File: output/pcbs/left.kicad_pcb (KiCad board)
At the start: 2 copper layers, 147 x 117.2 mm, 85 parts

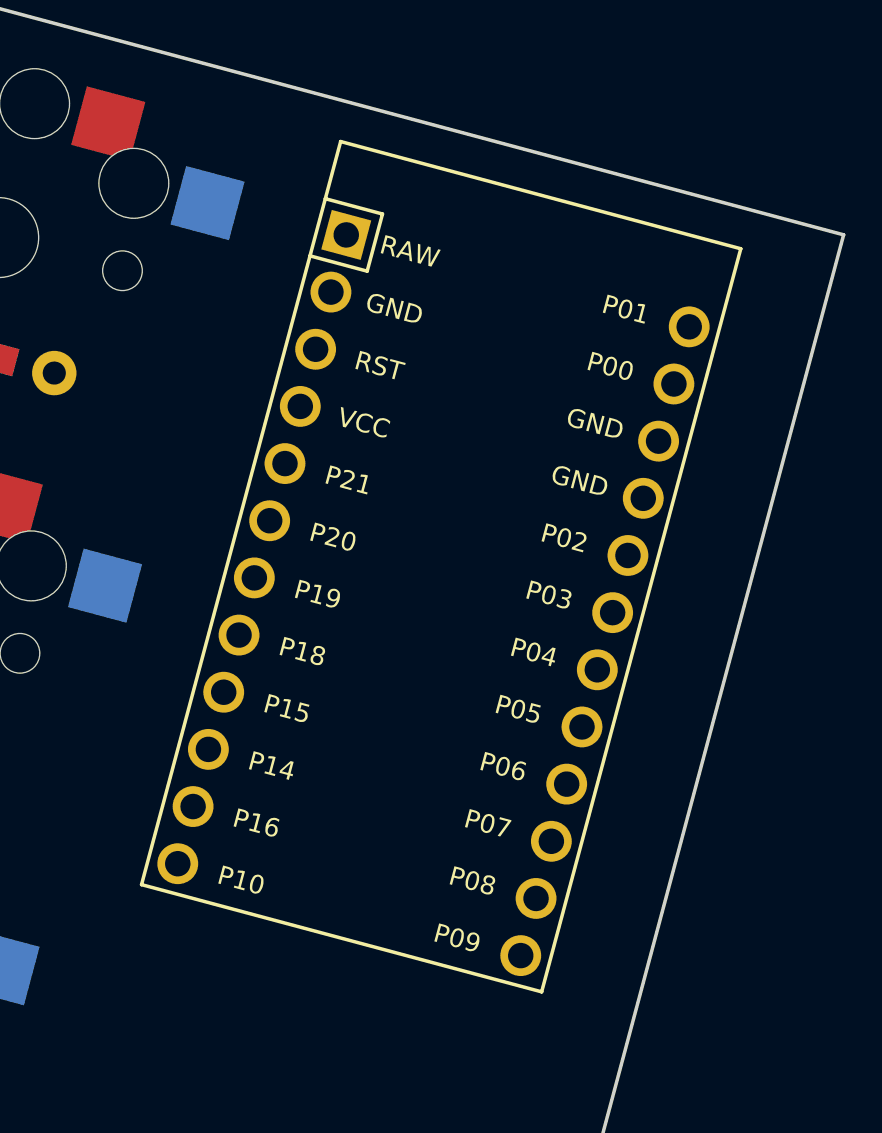
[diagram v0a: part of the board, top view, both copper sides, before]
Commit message: add nrf footprint
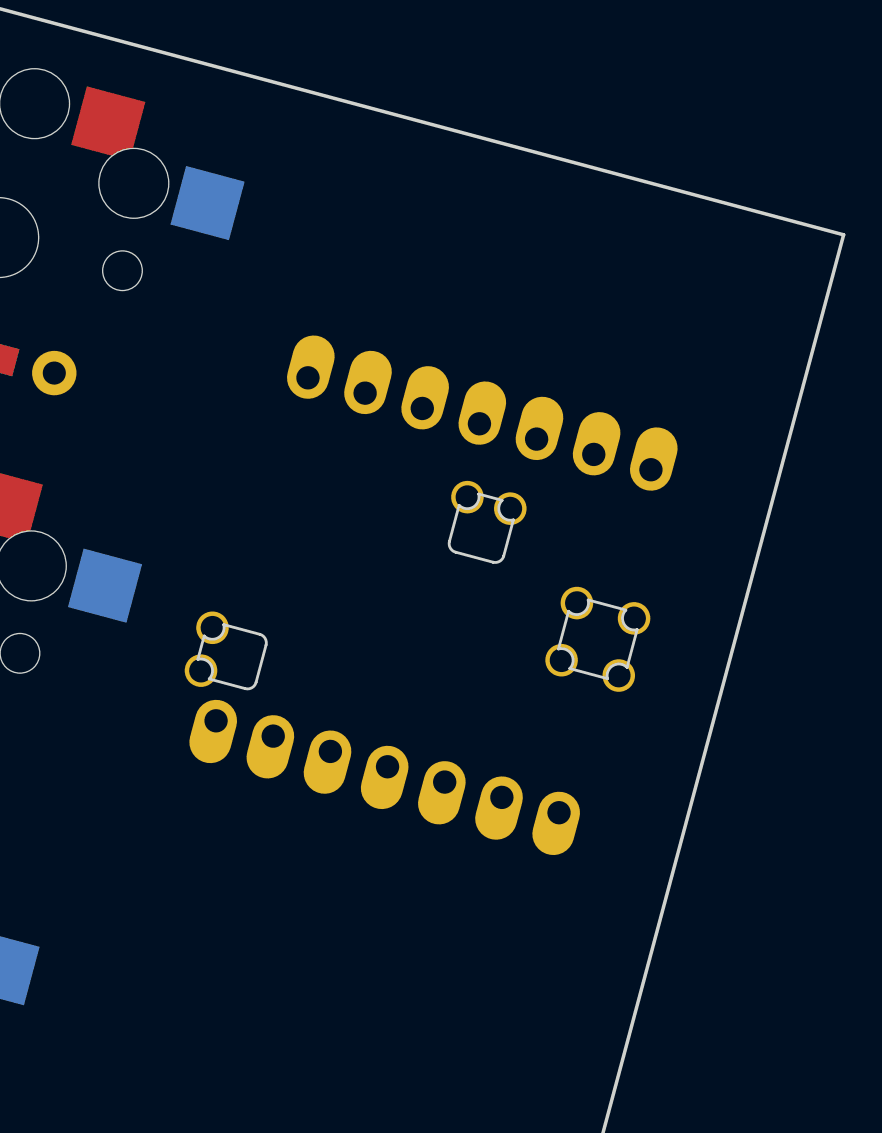
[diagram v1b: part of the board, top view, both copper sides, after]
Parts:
- MCU1: value (none) -> xiao-ble; footprint ProMicro -> XIAO-BLE
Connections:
- MCU1 pad 1: RAW -> P0
- MCU1 pad 10: P14 -> P9
- MCU1 pad 11: P16 -> P10
- MCU1 pad 12: P10 -> RAW3V3
- MCU1 pad 13: P1 -> GND
- MCU1 pad 14: P0 -> RAW5V
- MCU1 pad 15: GND -> SWCLK
- MCU1 pad 16: GND -> SWDIO
- MCU1 pad 17: P2 -> GND
- MCU1 pad 18: P3 -> RST
- MCU1 pad 19: P4 -> BAT_POS
- MCU1 pad 2: GND -> P1
- MCU1 pad 20: P5 -> BAT_NEG
- MCU1 pad 21: P6 -> NFC0
- MCU1 pad 22: P7 -> NFC1
- MCU1 pad 3: RST -> P2
- MCU1 pad 4: VCC -> P3
- MCU1 pad 5: P21 -> P4
- MCU1 pad 6: P20 -> P5
- MCU1 pad 7: P19 -> P6
- MCU1 pad 8: P18 -> P7
- MCU1 pad 9: P15 -> P8
